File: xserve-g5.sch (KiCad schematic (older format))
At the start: 17 parts, among them J1 SATA_Backplane_PWR, J10 FAN5_PWM, J11 FAN6_PWM, J12 FAN7_PWM, J2 FAN_LEFT, J3 FAN_RIGHT, J4 PWR_L, J5 PWR_R, J6 FAN1_PWM, J7 FAN2_PWM, J8 FAN3_PWM, J9 FAN4_PWM

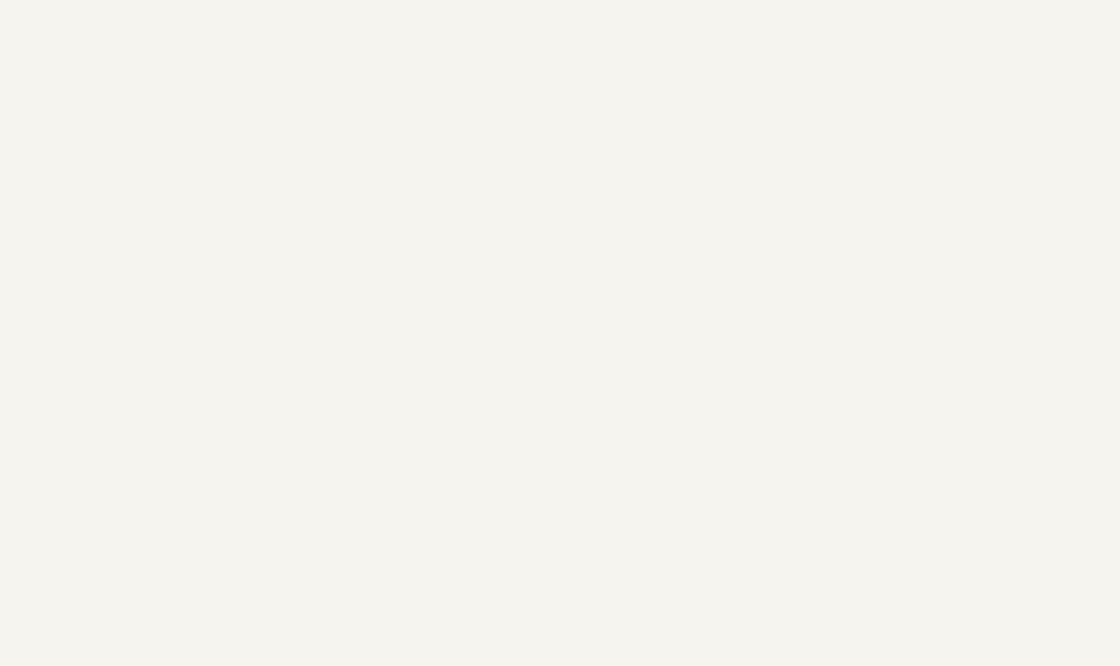
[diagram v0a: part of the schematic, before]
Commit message: updates
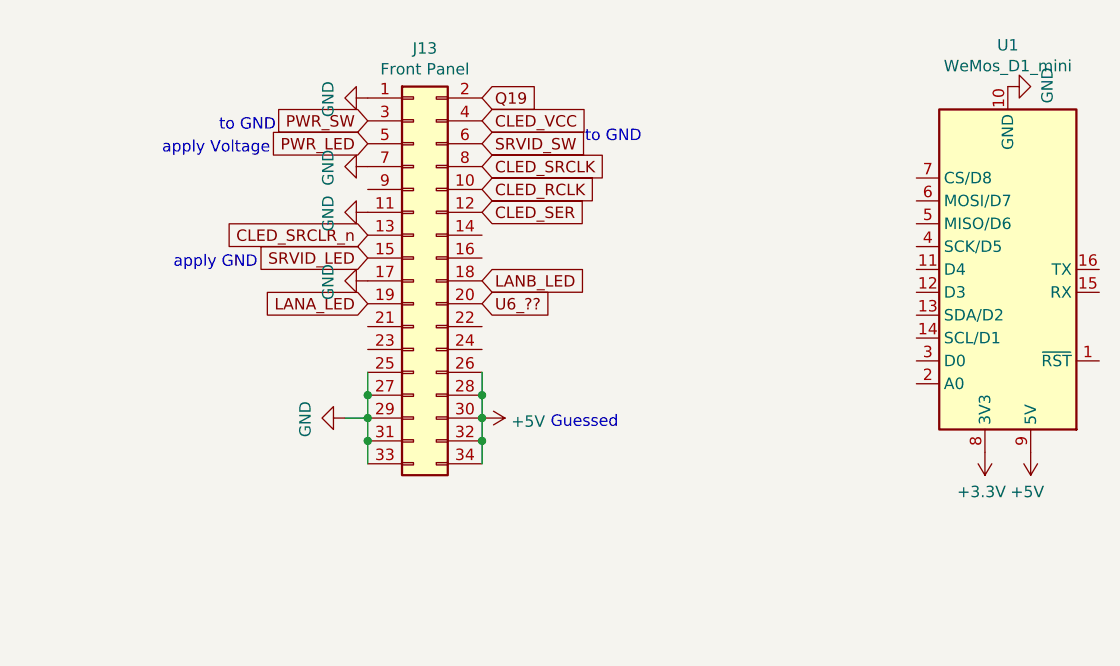
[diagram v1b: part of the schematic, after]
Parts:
- added J13: Front Panel, Connector_PinHeader_1.27mm:PinHeader_2x17_P1.27mm_Vertical, symbol Connector_Generic:Conn_02x17_Odd_Even
- added U1: WeMos_D1_mini, Module:WEMOS_D1_mini_light, symbol MCU_Module:WeMos_D1_mini
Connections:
- net +5V: now also J13.26 (Pin_26), J13.28 (Pin_28), J13.30 (Pin_30), J13.32 (Pin_32), J13.34 (Pin_34), U1.9 (5V)
- net GND: now also J13.1 (Pin_1), J13.11 (Pin_11), J13.17 (Pin_17), J13.25 (Pin_25), J13.27 (Pin_27), J13.29 (Pin_29), J13.31 (Pin_31), J13.33 (Pin_33), J13.7 (Pin_7), U1.10 (GND)
- new net +3V3: U1.8 (3V3)
- new net CLED_RCLK: J13.10 (Pin_10)
- new net CLED_SER: J13.12 (Pin_12)
- new net CLED_SRCLK: J13.8 (Pin_8)
- new net CLED_SRCLR_n: J13.13 (Pin_13)
- new net CLED_VCC: J13.4 (Pin_4)
- new net LANA_LED: J13.19 (Pin_19)
- new net LANB_LED: J13.18 (Pin_18)
- new net PWR_LED: J13.5 (Pin_5)
- new net PWR_SW: J13.3 (Pin_3)
- new net Q19: J13.2 (Pin_2)
- new net SRVID_LED: J13.15 (Pin_15)
- new net SRVID_SW: J13.6 (Pin_6)
- new net U6_??: J13.20 (Pin_20)
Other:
- note added: "Guessed"
- note added: "apply GND"
- note added: "apply Voltage"
- note added: "to GND"
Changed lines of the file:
@@
 Wire Notes Line
 	4850 550  550  550
+$Comp
+L power:GND #PWR0103
+U 1 1 5F39D41C
+P 6700 2300
+F 0 "#PWR0103" H 6700 2050 50  0001 C CNN
+F 1 "GND" H 6705 2127 50  0000 C CNN
+F 2 "" H 6700 2300 50  0001 C CNN
+F 3 "" H 6700 2300 50  0001 C CNN
+	1    6700 2300
+	0    1    1    0
+$EndComp
+$Comp
+L Connector_Generic:Conn_02x17_Odd_Even J13
+U 1 1 5F3A8D6B
+P 7000 1700
+F 0 "J13" H 7050 2717 50  0000 C CNN
+F 1 "Front Panel" H 7050 2626 50  0000 C CNN
+F 2 "Connector_PinHeader_1.27mm:PinHeader_2x17_P1.27mm_Vertical" H 7000 1700 50  0001 C CNN
+F 3 "~" H 7000 1700 50  0001 C CNN
+F 4 "Harwin M50-3551742" H 7000 1700 50  0001 C CNN "Part"
+	1    7000 1700
+	1    0    0    -1
+$EndComp
+$Comp
+L MCU_Module:WeMos_D1_mini U1
+U 1 1 5F3B1E0C
+P 9600 1650
+F 0 "U1" H 9600 669 50  0000 C CNN
+F 1 "WeMos_D1_mini" H 9600 760 50  0000 C CNN
+F 2 "Module:WEMOS_D1_mini_light" H 9600 500 50  0001 C CNN
+F 3 "https://wiki.wemos.cc/products:d1:d1_mini#documentation" H 7750 500 50  0001 C CNN
+	1    9600 1650
+	-1   0    0    1
+$EndComp
+$Comp
+L power:GND #PWR0121
+U 1 1 5F3C5F82
+P 9600 850
+F 0 "#PWR0121" H 9600 600 50  0001 C CNN
+F 1 "GND" H 9605 677 50  0000 C CNN
+F 2 "" H 9600 850 50  0001 C CNN
+F 3 "" H 9600 850 50  0001 C CNN
+	1    9600 850
+	0    -1   -1   0
+$EndComp
+Text GLabel 6800 1100 0    50   Input ~ 0
+PWR_LED
+Wire Wire Line
+	6800 2100 6800 2200
+Wire Wire Line
+	6800 2200 6800 2300
+Connection ~ 6800 2200
+Wire Wire Line
+	6800 2300 6800 2400
+Connection ~ 6800 2300
+Connection ~ 6800 2400
+Wire Wire Line
+	6800 2400 6800 2500
+Wire Wire Line
+	6700 2300 6800 2300
+Text GLabel 7300 1400 2    50   Input ~ 0
+CLED_SER
+Text GLabel 7300 1000 2    50   Input ~ 0
+CLED_VCC
+$Comp
+L power:GND #PWR?
+U 1 1 5F3CE2DC
+P 6800 900
+F 0 "#PWR?" H 6800 650 50  0001 C CNN
+F 1 "GND" H 6805 727 50  0000 C CNN
+F 2 "" H 6800 900 50  0001 C CNN
+F 3 "" H 6800 900 50  0001 C CNN
+	1    6800 900
+	0    1    1    0
+$EndComp
+$Comp
+L power:GND #PWR?
+U 1 1 5F3CEC27
+P 6800 1200
+F 0 "#PWR?" H 6800 950 50  0001 C CNN
+F 1 "GND" H 6805 1027 50  0000 C CNN
+F 2 "" H 6800 1200 50  0001 C CNN
+F 3 "" H 6800 1200 50  0001 C CNN
+	1    6800 1200
+	0    1    1    0
+$EndComp
+$Comp
+L power:GND #PWR?
+U 1 1 5F3CEED3
+P 6800 1400
+F 0 "#PWR?" H 6800 1150 50  0001 C CNN
+F 1 "GND" H 6805 1227 50  0000 C CNN
+F 2 "" H 6800 1400 50  0001 C CNN
+F 3 "" H 6800 1400 50  0001 C CNN
+	1    6800 1400
+	0    1    1    0
+$EndComp
+$Comp
+L power:GND #PWR?
+U 1 1 5F3CF6D7
+P 6800 1700
+F 0 "#PWR?" H 6800 1450 50  0001 C CNN
+F 1 "GND" H 6805 1527 50  0000 C CNN
+F 2 "" H 6800 1700 50  0001 C CNN
+F 3 "" H 6800 1700 50  0001 C CNN
+	1    6800 1700
+	0    1    1    0
+$EndComp
+Text GLabel 7300 1300 2    50   Input ~ 0
+CLED_RCLK
+Text GLabel 7300 1200 2    50   Input ~ 0
+CLED_SRCLK
+Text GLabel 6800 1500 0    50   Input ~ 0
+CLED_SRCLR_n
+Wire Wire Line
+	7300 2100 7300 2200
+Wire Wire Line
+	7300 2200 7300 2300
+Connection ~ 7300 2200
+Wire Wire Line
+	7300 2300 7300 2400
+Connection ~ 7300 2300
+Wire Wire Line
+	7300 2400 7300 2500
+Connection ~ 7300 2400
+$Comp
+L power:+5V #PWR?
+U 1 1 5F3D4B59
+P 7300 2300
+F 0 "#PWR?" H 7300 2150 50  0001 C CNN
+F 1 "+5V" V 7315 2428 50  0000 L CNN
+F 2 "" H 7300 2300 50  0001 C CNN
+F 3 "" H 7300 2300 50  0001 C CNN
+	1    7300 2300
+	0    1    1    0
+$EndComp
+$Comp
+L power:+5V #PWR?
+U 1 1 5F3D5D72
+P 9700 2450
+F 0 "#PWR?" H 9700 2300 50  0001 C CNN
+F 1 "+5V" H 9715 2623 50  0000 C CNN
+F 2 "" H 9700 2450 50  0001 C CNN
+F 3 "" H 9700 2450 50  0001 C CNN
+	1    9700 2450
+	-1   0    0    1
+$EndComp
+Text Notes 7600 2350 0    50   ~ 0
+Guessed
+Text GLabel 6800 1000 0    50   Input ~ 0
+PWR_SW
+Text Notes 6150 1050 0    50   ~ 0
+to GND
+Text GLabel 7300 1100 2    50   Input ~ 0
+SRVID_SW
+Text Notes 7750 1100 0    50   ~ 0
+to GND
+Text GLabel 6800 1600 0    50   Input ~ 0
+SRVID_LED
+Text Notes 5900 1150 0    50   ~ 0
+apply Voltage
+Text Notes 5950 1650 0    50   ~ 0
+apply GND
+Text GLabel 6800 1800 0    50   Input ~ 0
+LANA_LED
+Text GLabel 7300 1700 2    50   Input ~ 0
+LANB_LED
+$Comp
+L power:+3.3V #PWR?
+U 1 1 5F3DAB15
+P 9500 2450
+F 0 "#PWR?" H 9500 2300 50  0001 C CNN
+F 1 "+3.3V" H 9515 2623 50  0000 C CNN
+F 2 "" H 9500 2450 50  0001 C CNN
+F 3 "" H 9500 2450 50  0001 C CNN
+	1    9500 2450
+	-1   0    0    1
+$EndComp
+Text GLabel 7300 900  2    50   Input ~ 0
+Q19
+Text GLabel 7300 1800 2    50   Input ~ 0
+U6_??
 $EndSCHEMATC
